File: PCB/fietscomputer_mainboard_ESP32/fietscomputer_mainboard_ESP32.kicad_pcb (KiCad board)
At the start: 4 copper layers, 50 x 90 mm, 36 parts, among them J1 USB_C_Receptacle_USB2.0_14P, SW1 RESET1, SW2 BOOT1, SW3 GPS_RESET, SW4 PAGE_BUTTON, SW5 LAP_BUTTON, SW6 MAIN_BUTTON, SW7 ZOOM-_BUTTON, SW8 ZOOM+_BUTTON, U1 ESP32-S3-WROOM-1, U2 AMS1117-3.3, U3 L80-R, U5 IST8310

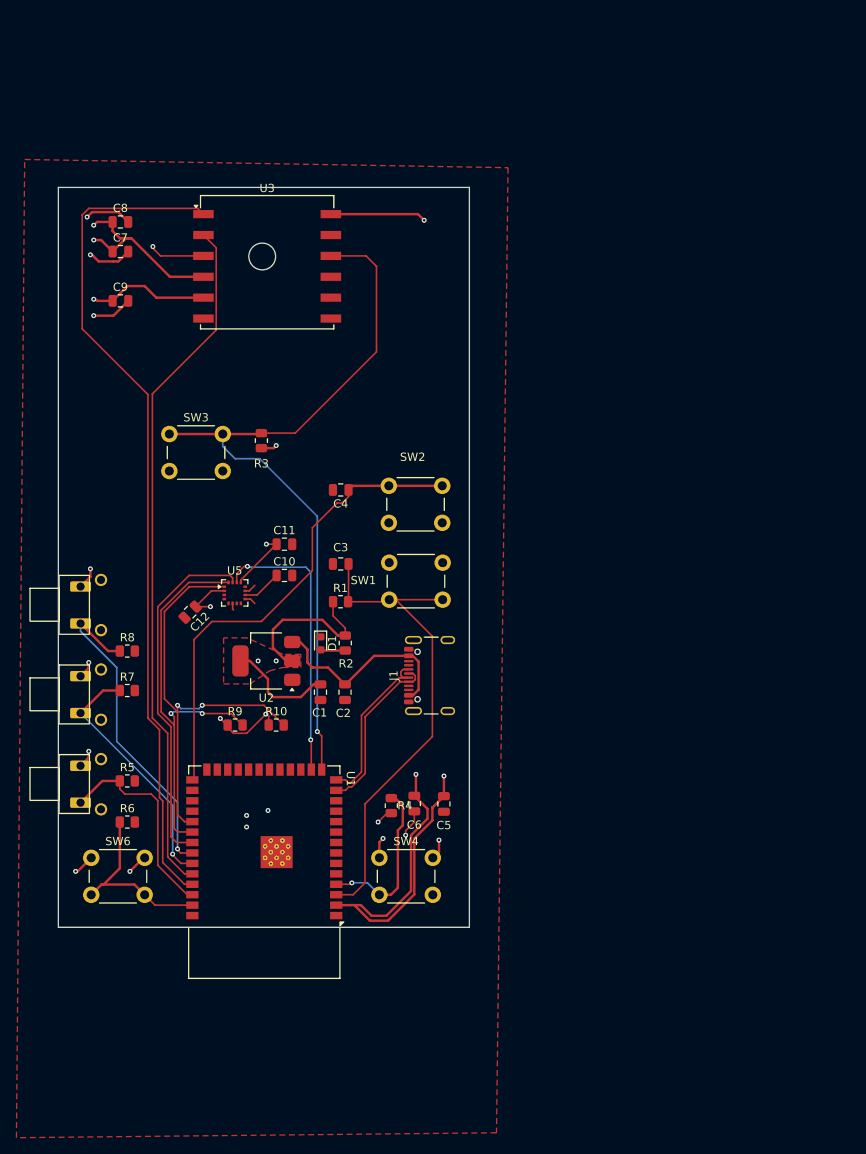
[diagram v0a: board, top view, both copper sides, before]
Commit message: new main
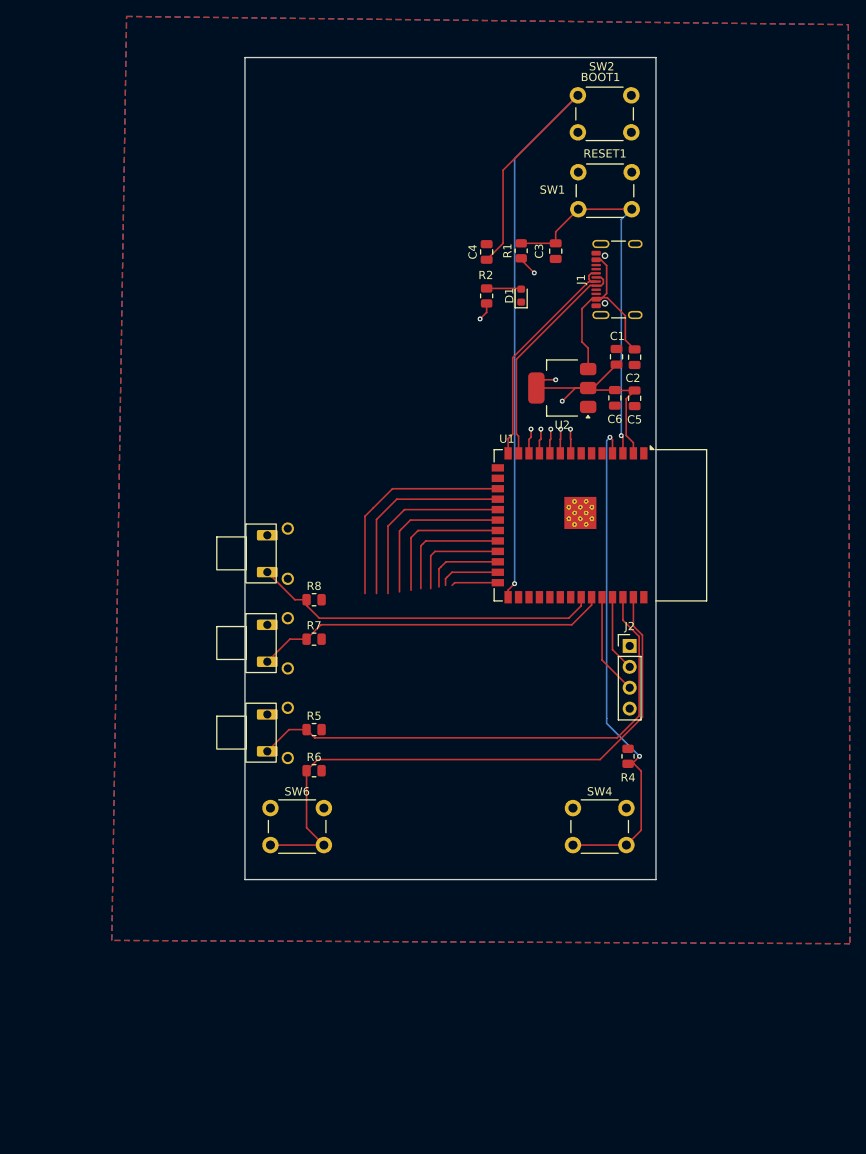
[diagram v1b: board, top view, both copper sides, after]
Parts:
- removed C10: 4.7uF, Capacitor_SMD:C_0805_2012Metric
- removed C11, C12: 0.1uF, Capacitor_SMD:C_0805_2012Metric
- removed C7: 10uF, Capacitor_SMD:C_0805_2012Metric
- removed C8, C9: 100uF, Capacitor_SMD:C_0805_2012Metric
- removed R10, R9: 4K7, Resistor_SMD:R_0805_2012Metric
- removed R3: 10K, Resistor_SMD:R_0805_2012Metric
- removed SW3: GPS_RESET, Button_Switch_THT:SW_PUSH_6mm
- removed U3: L80-R, RF_GPS:Quectel_L80-R
- removed U5: IST8310, Package_LGA:LGA-16_3x3mm_P0.5mm
- added J2: Conn_01x04_Pin, Connector_PinHeader_2.54mm:PinHeader_1x04_P2.54mm_Vertical, F.Cu at (191.2, 114.6)
- moved U1 58.8 mm to (187.7, 99.9), turned to -90 degrees
- moved C6 55.1 mm to (189.4, 84.4)
- moved C5 54.5 mm to (191.8, 84.5)
- moved C1 54.4 mm to (189.6, 79.4), turned to 90 degrees
- moved C2 53.9 mm to (191.8, 79.5)
- moved J1 53.3 mm to (190.8, 70.0)
- moved SW1 52.8 mm to (184.9, 57.0)
- moved SW2 52.8 mm to (191.4, 52.1)
- moved U2 49.0 mm to (183.0, 83.2)
- moved D1 48.8 mm to (178.0, 72.0), turned to 90 degrees
- moved R1 48.0 mm to (178.0, 66.5), turned to 90 degrees
- moved C3 46.2 mm to (182.2, 66.5), turned to -90 degrees
- moved R2 45.6 mm to (173.8, 72.0), turned to 90 degrees
- moved C4 34.0 mm to (173.8, 66.7), turned to 90 degrees
- moved R4 29.4 mm to (191.0, 128.0), turned to 90 degrees
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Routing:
- net +3.3V: track 164.9 -> 36.7 mm, vias 19 -> 4
- net RX_GPS: track 102.9 -> 9.34 mm
- net GPS_RESET: track 93.4 -> 0.00 mm, vias 1 -> 0
- net TX_GPS: track 84.1 -> 12.4 mm
- net MAIN_BUTTON: track 22.5 -> 75.0 mm
- net I2C_SCL: track 51.1 -> 0.00 mm, vias 2 -> 0
- net I2C_SDA: track 50.2 -> 0.00 mm, vias 2 -> 0
- net GND: track 43.6 -> 0.00 mm, vias 10 -> 0
- net DATA_READY_COMP: track 42.9 -> 0.00 mm
- net PAGE_BUTTON: track 20.5 -> 62.7 mm, vias 1 -> 2
- net LAP_BUTTON: track 25.6 -> 63.1 mm
- net COMPASS_RESET: track 35.2 -> 0.00 mm, vias 2 -> 0
- net IO1: track 58.6 -> 89.2 mm, vias 0 -> 1
- net unconnected-(U1-IO9-Pad17): track 0.00 -> 26.9 mm
- net unconnected-(U1-IO10-Pad18): track 0.00 -> 24.8 mm
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- added copper zone on B.Cu, net GND
- removed copper zone on F.Cu, net +3.3V
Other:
- board size 50 x 90 mm -> 50 x 100 mm
